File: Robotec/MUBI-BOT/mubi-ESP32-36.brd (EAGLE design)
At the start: 100 x 50.2 mm, 22 parts, among them IC1 L293D, IC2 7805T

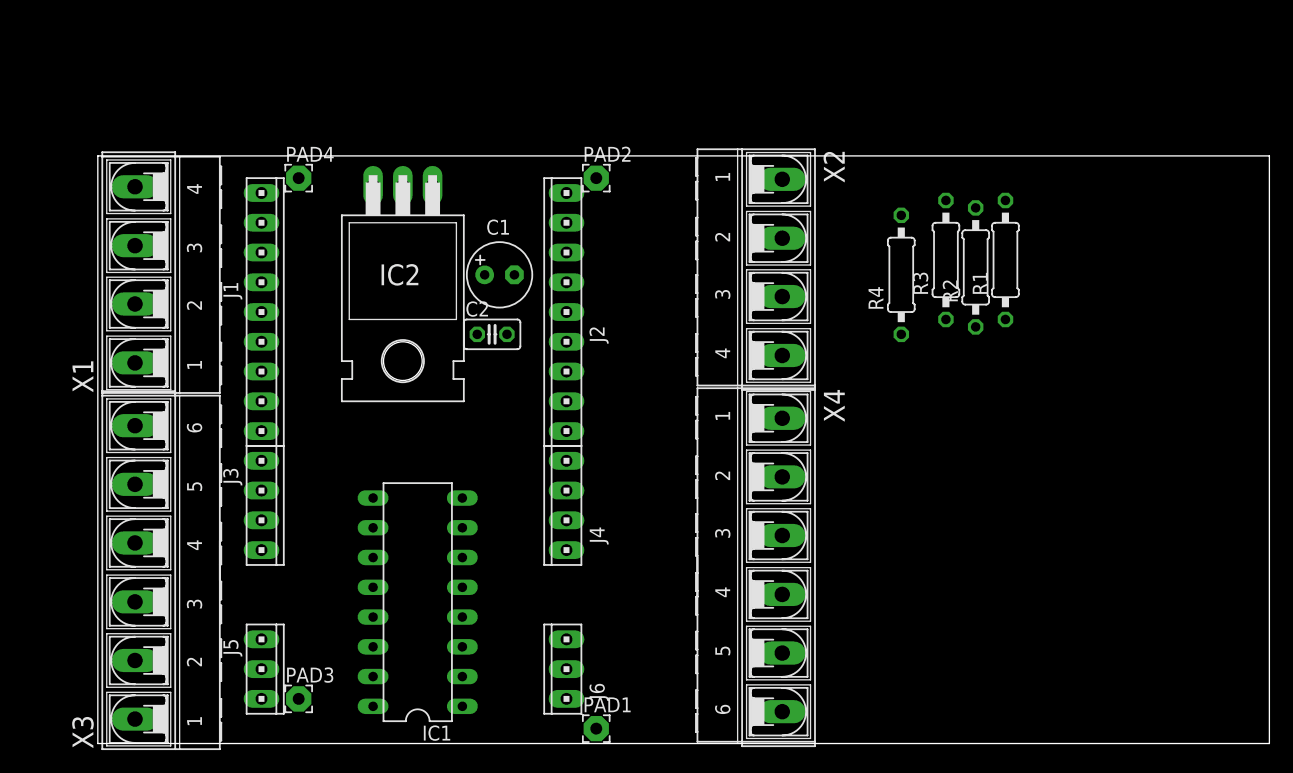
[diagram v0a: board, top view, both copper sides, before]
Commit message: update MUBI-BOT
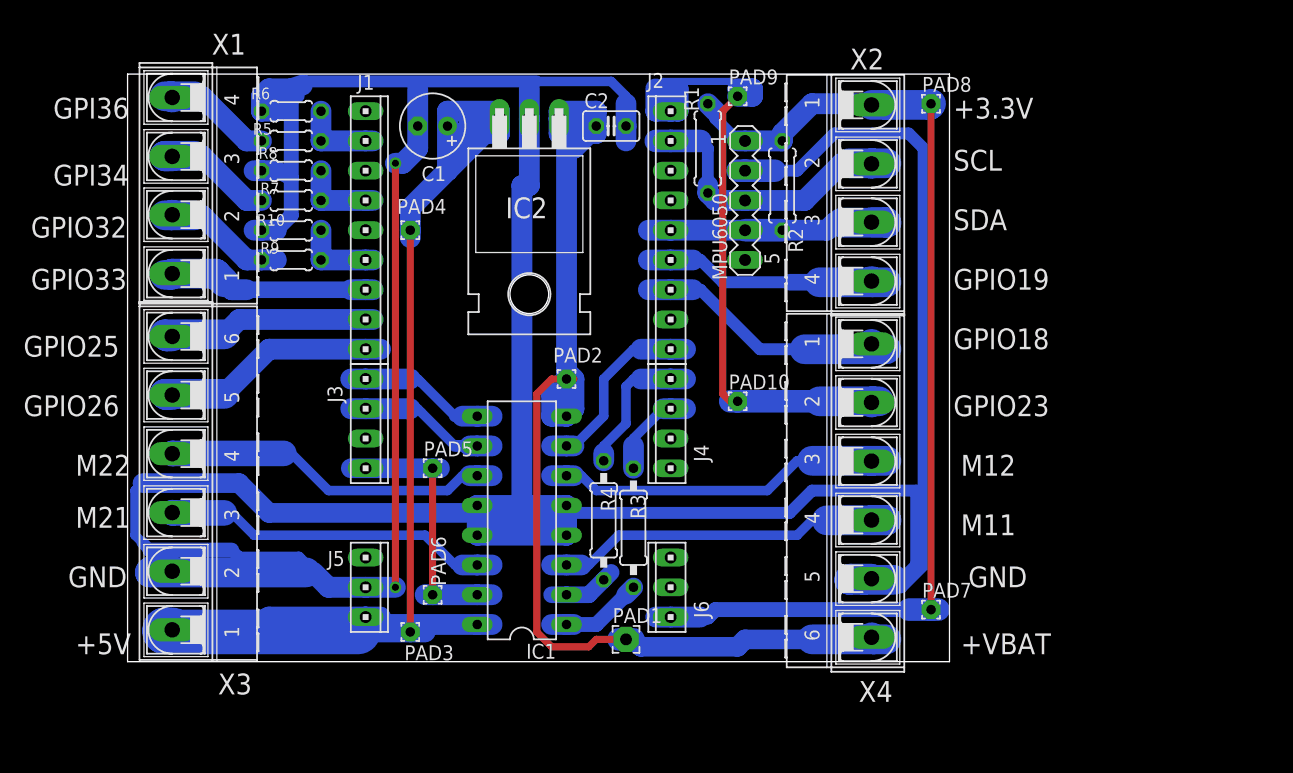
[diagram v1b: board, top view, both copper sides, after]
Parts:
- added MPU6050: (no value), con-lstb:MA05-1
- added PAD10, PAD5, PAD6, PAD7, PAD8, PAD9: WIREPAD1,6/0,8, wirepad:1,6/0,8
- added R10, R6, R8: 10K, resistor:0204/5
- added R5, R7, R9: 5K6, resistor:0204/5
- PAD2, PAD3, PAD4: value WIREPAD2,15/1,0 -> WIREPAD1,6/0,8; device wirepad:2,15/1,0 -> wirepad:1,6/0,8
- R1, R2: value (none) -> 4K7; device resistor:0207/10 -> rcl:0207/7
- R3, R4: value (none) -> 1
- moved R3 35.1 mm to (45.7, 18.4)
- moved R4 32.9 mm to (43.2, 19.1)
- moved R1 27.1 mm to (52.1, 50.8)
- moved C2 20.5 mm to (43.8, 52.7)
- moved R2 17.9 mm to (58.4, 47.6)
- moved PAD2 17.3 mm to (40.0, 31.1)
- moved C1 13.9 mm to (28.6, 52.7), turned to 180 degrees
- moved IC2 12.2 mm to (36.8, 43.2)
- moved IC1 11.3 mm to (36.2, 19.1)
- moved J6 11.3 mm to (48.9, 13.3)
- moved J1 11.3 mm to (22.9, 43.8)
- moved J2 11.3 mm to (48.9, 43.8)
- moved J3 11.3 mm to (22.9, 27.3)
- moved J4 11.3 mm to (48.9, 27.3)
- moved J5 11.3 mm to (22.9, 13.3)
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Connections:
- removed net GND1: IC1.4
- removed net GND2: IC1.5
- removed net GND3: IC1.13
- removed net GND4: IC1.12
- removed net VCC1: IC1.16
- removed net VCC2: IC1.8
- new net +3.3V: J6.3, MPU6050.1, PAD7.1, PAD8.1, R1.2, R2.2, X2.1
- new net +5V: C1.+, IC1.16, IC2.3, J5.1, PAD3.1, PAD4.1, X3.1
- new net +VBAT: C2.1, IC1.8, IC2.1, PAD1.1, PAD2.1, X4.6
- new net CM11: IC1.2, R4.1
- new net CM12: IC1.7, J2.9
- new net CM21: IC1.15, J3.1, PAD5.1, PAD6.1
- new net CM22: IC1.10, J3.3
- new net ENAM1: IC1.1, R3.1
- new net ENAM2: IC1.9, J3.4
- new net GND: C1.-, C2.2, IC1.12, IC1.13, IC1.4, IC1.5, IC2.2, J5.2, MPU6050.2, R10.2, R6.2, R8.2, X3.2, X4.5
- new net GPI34: J1.6, R7.2, R8.1
- new net GPI36: J1.8, R5.2, R6.1
- new net GPIO18: J2.7, X4.1
- new net GPIO19: J2.6, X2.4
- new net GPIO23: J2.1, PAD10.1, PAD9.1, X4.2
- new net GPIO25: J1.2, X3.6
- new net GPIO26: J1.1, X3.5
- new net GPIO32: J1.4, R10.1, R9.2
- new net GPIO33: J1.3, X1.1
- new net M11: IC1.3, X4.4
- new net M12: IC1.6, X4.3
- new net M21: IC1.14, X3.3
- new net M22: IC1.11, X3.4
- new net N$3: R5.1, X1.4
- new net N$5: R7.1, X1.3
- new net N$8: R9.1, X1.2
- new net SCL: J2.2, MPU6050.3, R1.1, X2.2
- new net SDA: J2.5, MPU6050.4, R2.1, X2.3
- net N$1: now also J4.2, R3.2; no longer PAD1.1, PAD2.1
- net N$2: now also J4.1, R4.2; no longer PAD3.1, PAD4.1
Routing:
- net GND: track 0.00 -> 373.5 mm, vias 0 -> 2
- net +5V: track 0.00 -> 120.0 mm
- net +VBAT: track 0.00 -> 105.4 mm, vias 0 -> 1
- net +3.3V: track 0.00 -> 91.4 mm
- net GPIO23: track 0.00 -> 59.2 mm
- net M11: track 0.00 -> 31.4 mm
- net M12: track 0.00 -> 30.2 mm
- net M22: track 0.00 -> 29.2 mm
- net M21: track 0.00 -> 29.2 mm
- net SCL: track 0.00 -> 25.4 mm
- net CM21: track 0.00 -> 25.4 mm
- net GPIO18: track 0.00 -> 23.1 mm
- net SDA: track 0.00 -> 21.9 mm
- net GPIO19: track 0.00 -> 21.3 mm
- net GPIO26: track 0.00 -> 20.7 mm
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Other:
- board size 100 x 50.2 mm -> 70.2 x 50.2 mm
- board text added: "+3.3V"
- board text added: "+5V"
- board text added: "+VBAT"
- board text added: "GND"
- board text added: "GPI34"
- board text added: "GPI36"
- board text added: "GPIO18"
- board text added: "GPIO19"
- board text added: "GPIO23"
- board text added: "GPIO25"
- board text added: "GPIO26"
- board text added: "GPIO32"
- board text added: "GPIO33"
- board text added: "M11"
- board text added: "M12"
- board text added: "M21"
- board text added: "M22"
- board text added: "SCL"
- board text added: "SDA"
